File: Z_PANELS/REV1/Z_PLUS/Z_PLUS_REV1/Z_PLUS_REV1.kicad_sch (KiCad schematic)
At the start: 1 part, among them J1 F3311A7H121014E200

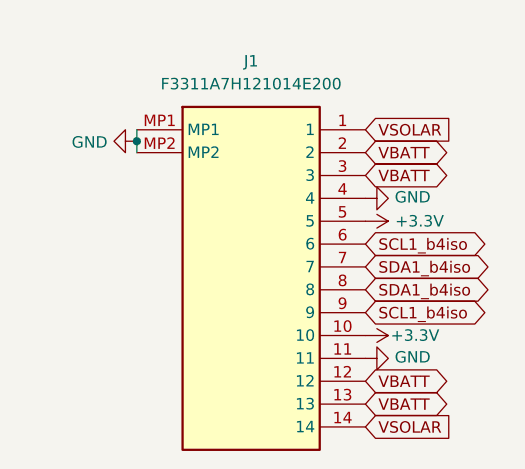
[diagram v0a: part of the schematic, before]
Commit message: made changes to Z plus board
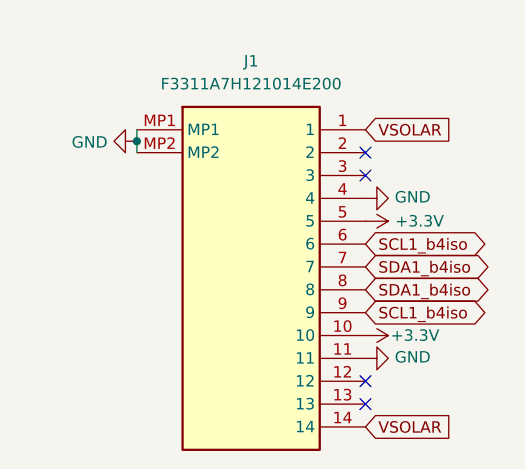
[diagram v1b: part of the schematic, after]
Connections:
- removed net VBATT: J1.12, J1.13, J1.2, J1.3
- no-connect marks 0 -> 4
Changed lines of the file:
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@@
   (junction (at 159.766 53.594) (diameter 0) (color 0 0 0 0)
   )
+  (no_connect (at 185.166 54.864))
+  (no_connect (at 185.166 57.404))
+  (no_connect (at 185.166 82.804))
+  (no_connect (at 185.166 80.264))
   (wire (pts (xy 159.766 53.594) (xy 159.766 54.864))
     (stroke (width 0) (type default))
@@
     )
   )
-  (global_label "VBATT" (shape bidirectional) (at 185.166 80.264 0)
-    (effects (font (size 1.27 1.27)) (justify left))
-    (property "Intersheetrefs" "${INTERSHEET_REFS}" (at 185.166 80.264 0)
-      (effects (font (size 1.27 1.27)) hide)
-    )
-  )
-  (global_label "VBATT" (shape bidirectional) (at 185.166 82.804 0)
-    (effects (font (size 1.27 1.27)) (justify left))
-    (property "Intersheetrefs" "${INTERSHEET_REFS}" (at 185.166 82.804 0)
-      (effects (font (size 1.27 1.27)) hide)
-    )
-  )
-  (global_label "VBATT" (shape bidirectional) (at 185.166 57.404 0)
-    (effects (font (size 1.27 1.27)) (justify left))
-    (property "Intersheetrefs" "${INTERSHEET_REFS}" (at 185.166 57.404 0)
-      (effects (font (size 1.27 1.27)) hide)
-    )
-  )
   (global_label "SDA1_b4iso" (shape bidirectional) (at 185.166 67.564 0)
     (effects (font (size 1.27 1.27)) (justify left))
@@
       (effects (font (size 1.27 1.27)) hide)
     )
-  )
-  (global_label "VBATT" (shape bidirectional) (at 185.166 54.864 0)
-    (effects (font (size 1.27 1.27)) (justify left))
-    (property "Intersheetrefs" "${INTERSHEET_REFS}" (at 185.166 54.864 0)
-      (effects (font (size 1.27 1.27)) hide)
-    )
